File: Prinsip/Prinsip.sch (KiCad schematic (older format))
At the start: 26 parts

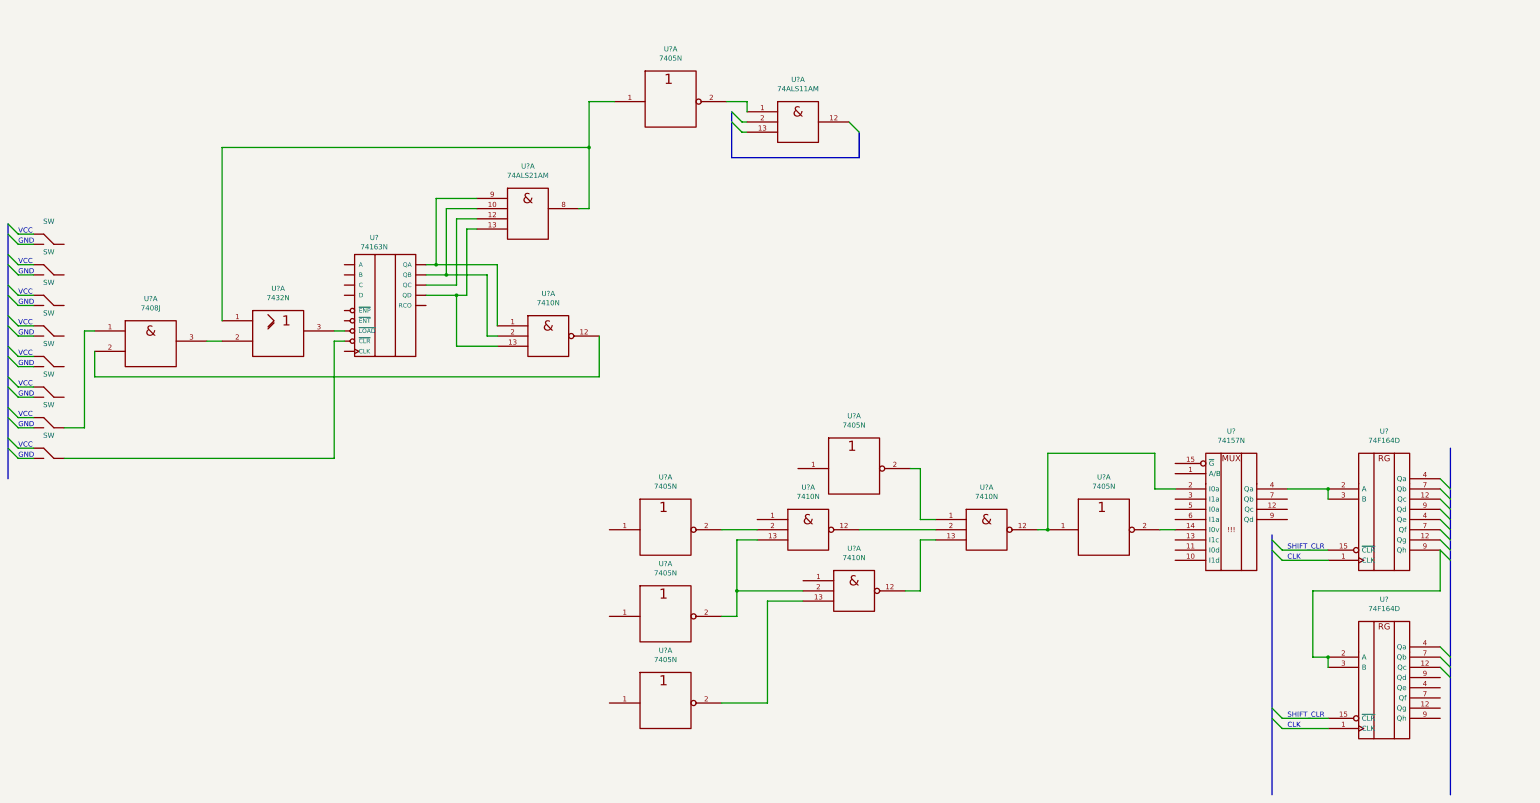
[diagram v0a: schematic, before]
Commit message: Updated
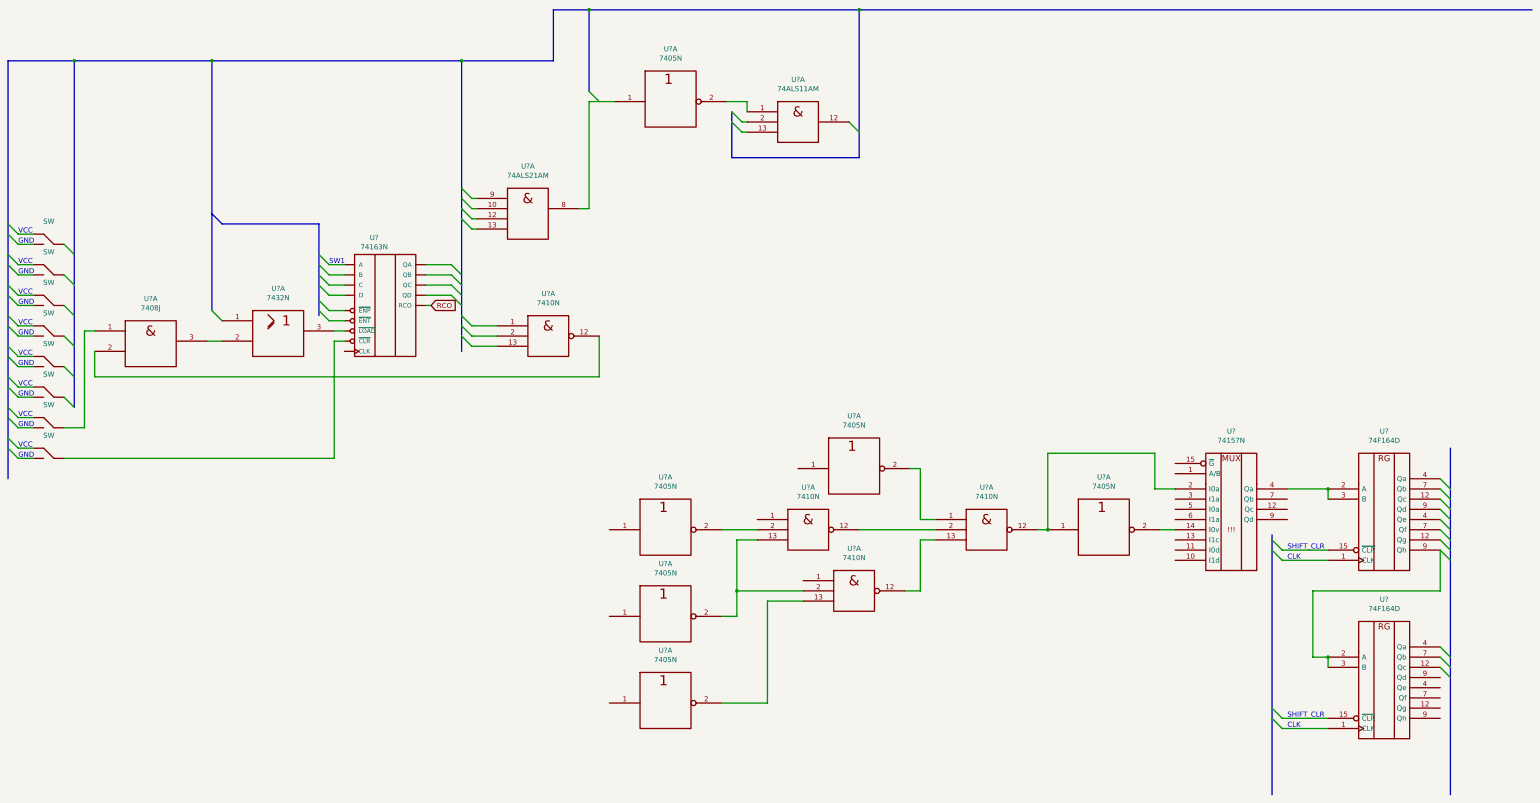
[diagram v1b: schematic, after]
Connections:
- net RCO: now reaches U?.~ (~LOAD)
- net at U?.12: no longer U?.~ (~LOAD)
- net at U?.~: no longer U?.~ (~LOAD)
- net at U?.1, U?.8: no longer U?.1
- net at U?.9 (Qh): now also U?.2 (A), U?.3 (B)
- new net: U?.~, U?.~ (~LOAD)
- now unconnected: U?.1, U?.10, U?.13, U?.13, U?.2, U?.9
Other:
- note added: "SW1"
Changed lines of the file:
@@
 	8350 1300 8350 1400
 Wire Bus Line
-	9450 1850 9450 1600
-Wire Bus Line
 	8200 1850 9450 1850
-Entry Wire Line
-	9350 1500 9450 1600
-Wire Wire Line
-	5700 2250 5300 2250
-Wire Wire Line
-	5300 2250 5300 2900
-Wire Wire Line
-	5300 2900 5200 2900
-Wire Wire Line
-	5200 3000 5400 3000
-Wire Wire Line
-	5400 3000 5400 2350
-Wire Wire Line
-	5400 2350 5700 2350
-Wire Wire Line
-	5700 2450 5500 2450
-Wire Wire Line
-	5500 2450 5500 3100
-Wire Wire Line
-	5500 3100 5200 3100
-Wire Wire Line
-	5200 3200 5500 3200
-Wire Wire Line
-	5600 3200 5600 2550
-Wire Wire Line
-	5600 2550 5700 2550
 Wire Wire Line
 	6700 2350 6800 2350
 Wire Wire Line
-	6800 2350 6800 1750
-Wire Wire Line
-	6800 1300 7050 1300
-Wire Wire Line
-	5300 2900 5900 2900
-Wire Wire Line
-	5900 2900 5900 3500
-Connection ~ 5300 2900
-Wire Wire Line
-	5400 3000 5800 3000
-Wire Wire Line
-	5800 3000 5800 3600
-Wire Wire Line
-	5800 3600 5900 3600
-Connection ~ 5400 3000
-Wire Wire Line
-	5500 3200 5500 3700
-Wire Wire Line
-	5500 3700 5900 3700
-Connection ~ 5500 3200
-Wire Wire Line
-	5500 3200 5600 3200
-Wire Wire Line
 	4300 3550 4400 3550
 Wire Wire Line
 	3050 3650 3200 3650
-Wire Wire Line
-	3200 3450 3200 1750
-Wire Wire Line
-	3200 1750 6800 1750
-Connection ~ 6800 1750
-Wire Wire Line
-	6800 1750 6800 1300
 $Comp
 L Prinsip:SW U?
@@
 	4300 3650 4400 3650
 Wire Bus Line
+	1100 900  1750 900
+Wire Bus Line
+	6450 900  6450 400
+Wire Bus Line
+	6450 400  6800 400
+Connection ~ 9450 400
+Wire Bus Line
+	9450 400  16050 400
+Entry Wire Line
+	9350 1500 9450 1600
+Connection ~ 1750 900
+Wire Bus Line
+	1750 900  3100 900
+Entry Wire Line
+	1650 2700 1750 2800
+Entry Wire Line
+	1650 3000 1750 3100
+Entry Wire Line
+	1650 3300 1750 3400
+Entry Wire Line
+	1650 3600 1750 3700
+Entry Wire Line
+	1650 3900 1750 4000
+Entry Wire Line
+	1650 4200 1750 4300
+Wire Wire Line
+	6800 1300 6800 2350
+Connection ~ 3100 900
+Wire Bus Line
+	3100 900  5550 900
+Entry Wire Line
+	3100 3350 3200 3450
+Wire Bus Line
+	6800 400  6800 1200
+Connection ~ 6800 400
+Wire Bus Line
+	6800 400  9450 400
+Entry Wire Line
+	6800 1200 6900 1300
+Entry Bus Bus
+	3100 2400 3200 2500
+Wire Bus Line
+	3200 2500 4150 2500
+Entry Wire Line
+	4150 2800 4250 2900
+Entry Wire Line
+	4150 2900 4250 3000
+Entry Wire Line
+	4150 3000 4250 3100
+Entry Wire Line
+	4150 3100 4250 3200
+Entry Wire Line
+	4150 3250 4250 3350
+Entry Wire Line
+	4150 3350 4250 3450
+Wire Wire Line
+	4250 2900 4400 2900
+Text Notes 4250 2900 0    50   ~ 0
+SW1
+Wire Wire Line
+	4250 3000 4400 3000
+Wire Wire Line
+	4250 3100 4400 3100
+Wire Wire Line
+	4400 3200 4250 3200
+Wire Wire Line
+	4250 3350 4400 3350
+Wire Wire Line
+	4400 3450 4250 3450
+Connection ~ 5550 900
+Wire Bus Line
+	5550 900  6450 900
+Wire Wire Line
+	5200 2900 5450 2900
+Entry Wire Line
+	5450 2900 5550 3000
+Wire Wire Line
+	5200 3000 5450 3000
+Entry Wire Line
+	5450 3000 5550 3100
+Wire Wire Line
+	5200 3100 5450 3100
+Entry Wire Line
+	5450 3100 5550 3200
+Wire Wire Line
+	5200 3200 5450 3200
+Entry Wire Line
+	5450 3200 5550 3300
+Text GLabel 5250 3300 2    50   Input ~ 0
+RCO
+Wire Wire Line
+	5200 3300 5250 3300
+Wire Wire Line
+	5650 2250 5700 2250
+Wire Wire Line
+	5650 2350 5700 2350
+Entry Wire Line
+	5550 2150 5650 2250
+Entry Wire Line
+	5550 2250 5650 2350
+Entry Wire Line
+	5550 2350 5650 2450
+Entry Wire Line
+	5550 2450 5650 2550
+Wire Wire Line
+	5650 2450 5700 2450
+Wire Wire Line
+	5700 2550 5650 2550
+Wire Wire Line
+	5650 3500 5900 3500
+Wire Wire Line
+	5900 3600 5650 3600
+Wire Wire Line
+	5650 3700 5900 3700
+Wire Bus Line
+	3100 900  3100 3350
+Wire Wire Line
+	6800 1300 7050 1300
+Wire Bus Line
+	9450 400  9450 1850
+Wire Bus Line
 	8200 1400 8200 1850
 Wire Bus Line
 	13500 5550 13500 8100
 Wire Bus Line
+	1750 900  1750 4300
+Wire Bus Line
+	4150 2500 4150 3400
+Wire Bus Line
+	5550 900  5550 3750
+Wire Bus Line
 	15250 4700 15250 8100
 Wire Bus Line
-	1100 2500 1100 5000
+	1100 900  1100 5000
+Entry Wire Line
+	5550 3400 5650 3500
+Entry Wire Line
+	5550 3500 5650 3600
+Entry Wire Line
+	5550 3600 5650 3700
 $EndSCHEMATC
